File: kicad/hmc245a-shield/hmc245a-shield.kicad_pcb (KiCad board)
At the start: 2 copper layers, 68.6 x 53.3 mm, 14 parts, among them IC1 HMC245AQS16E, J1 Power, J2 Digital/PWM, J3 Analog, J4 Digital/PWM, J5 Conn_Coaxial, J6 Conn_Coaxial, J7 Conn_Coaxial, J8 Conn_Coaxial

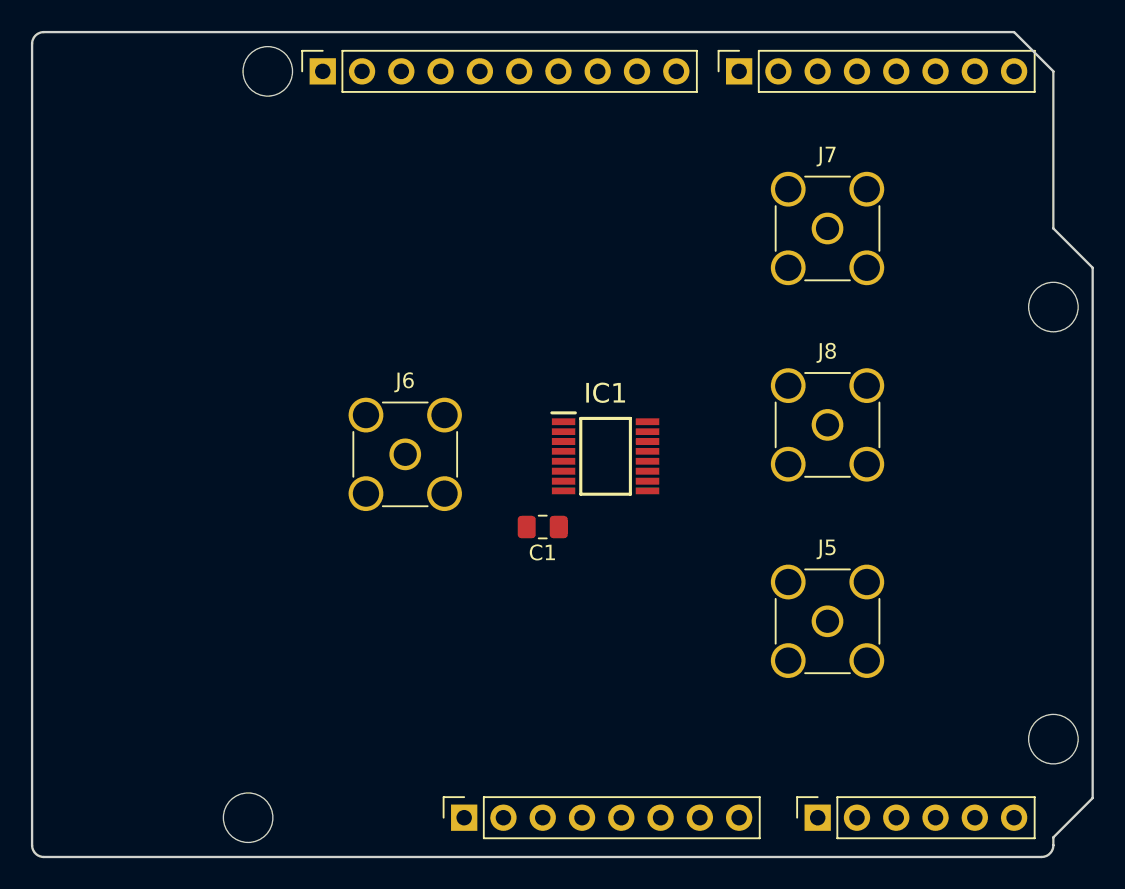
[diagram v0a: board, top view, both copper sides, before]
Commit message: パターンをひいた
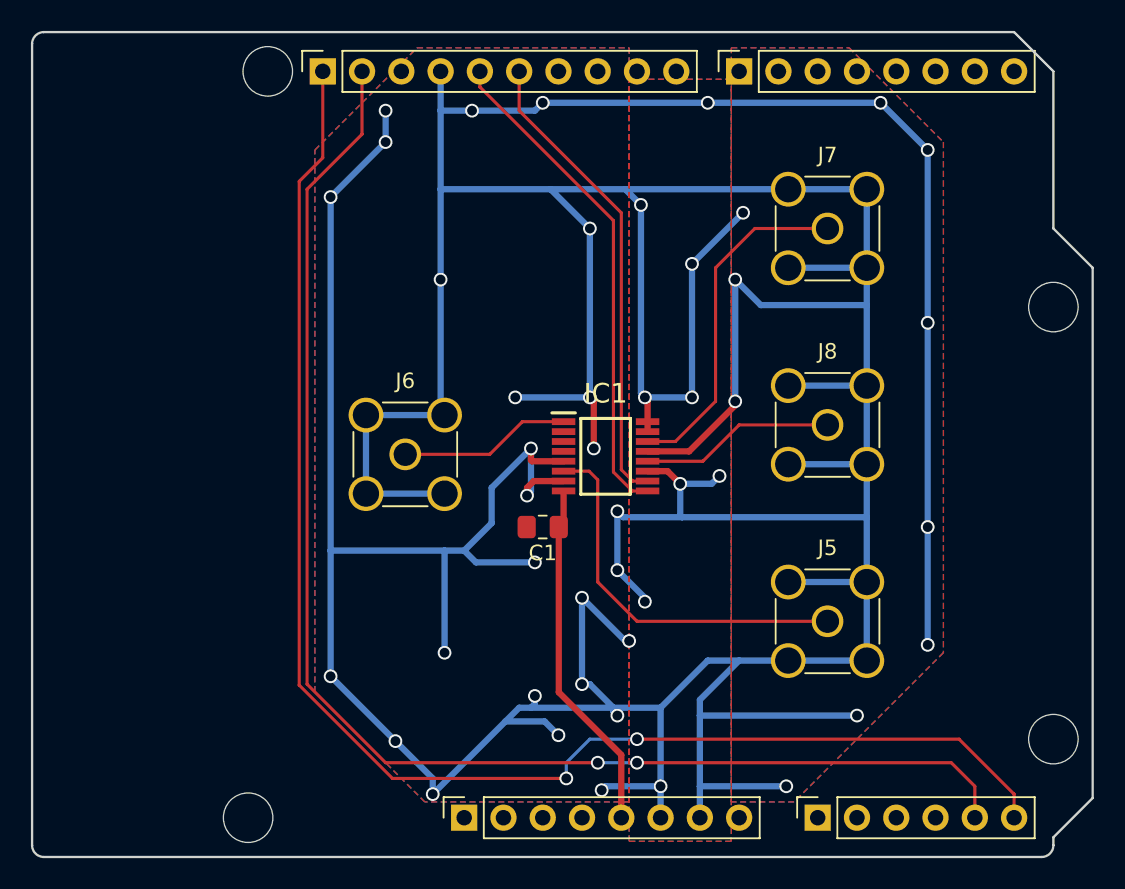
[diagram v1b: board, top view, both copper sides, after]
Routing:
- net GND: track 0.00 -> 464.2 mm, vias 0 -> 45
- net /SCL/A5: track 0.00 -> 93.7 mm, vias 0 -> 2
- net /SDA/A4: track 0.00 -> 89.0 mm, vias 0 -> 2
- net /13: track 0.00 -> 32.2 mm
- net /12: track 0.00 -> 30.5 mm
- net Net-(IC1-Pad6): track 0.00 -> 25.0 mm
- net +5V: track 0.00 -> 22.9 mm
- net Net-(IC1-Pad14): track 0.00 -> 22.4 mm
- net Net-(IC1-Pad12): track 0.00 -> 12.6 mm
- net Net-(IC1-Pad1): track 0.00 -> 11.1 mm
- added copper zone on B.Cu, net GND
- added copper zone on F.Cu, net GND
